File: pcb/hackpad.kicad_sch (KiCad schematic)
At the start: 39 parts, among them SW1 SW_Push, SW11 RotaryEncoder_Switch, SW2 SW_Push, SW3 SW_Push, SW4 SW_Push, SW6 SW_Push, SW7 SW_Push, SW8 SW_Push, SW9 SW_Push, U1 XIAO-RP2040-DIP

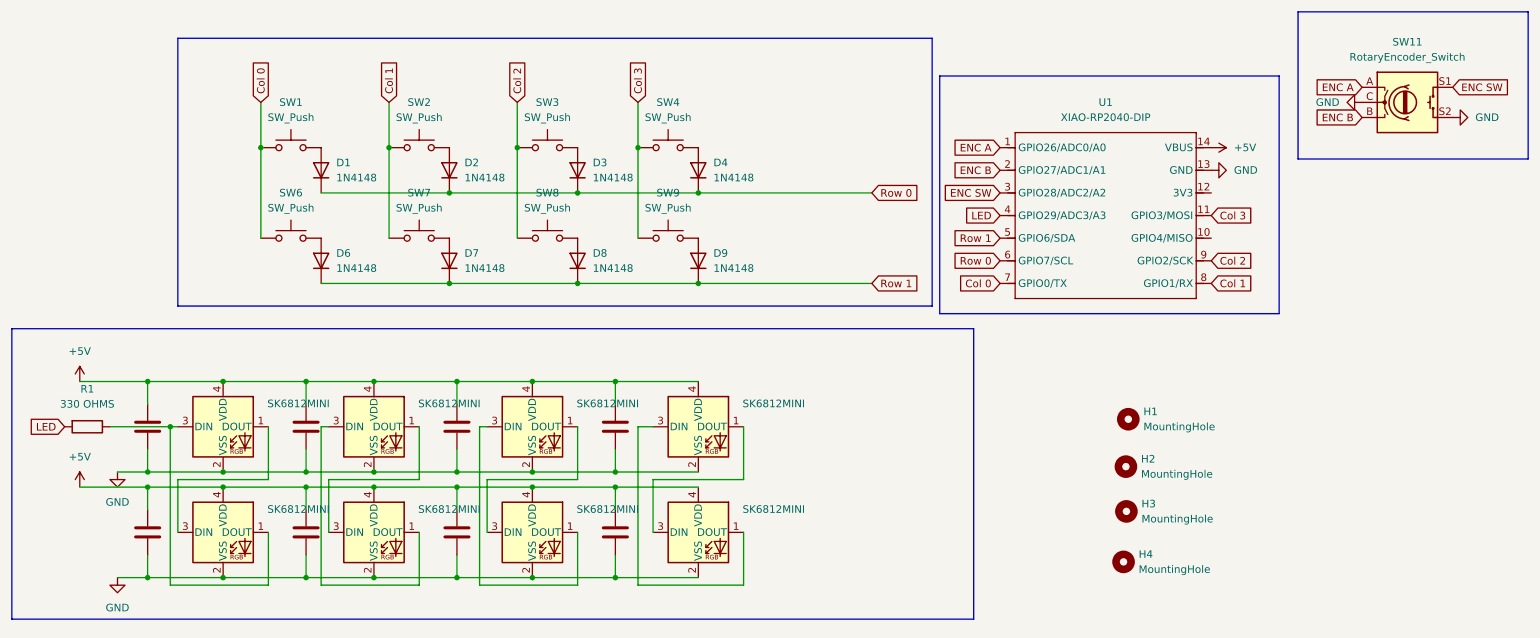
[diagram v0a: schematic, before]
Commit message: updated pcb final
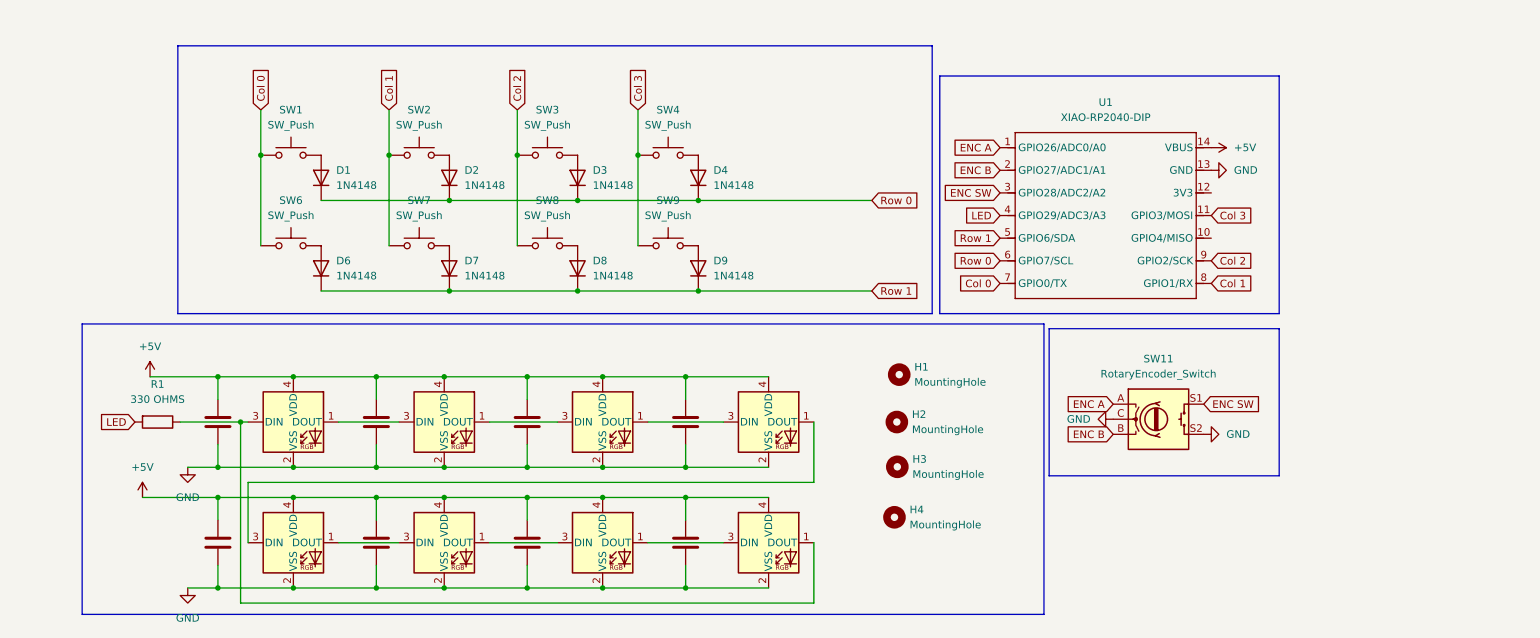
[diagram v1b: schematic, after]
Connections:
- net at D19.1 (DOUT): now also D14.3 (DIN); no longer D17.3 (DIN)
- net at D19.3 (DIN): now also D13.1 (DOUT); no longer D17.1 (DOUT)
- net at D11.1 (DOUT): now also D12.3 (DIN); no longer D14.3 (DIN)
- net at D11.3 (DIN), R1.1: now also D17.1 (DOUT); no longer D14.1 (DOUT)
- net at D16.1 (DOUT): now also D17.3 (DIN); no longer D13.3 (DIN)
- net at D16.3 (DIN): now also D15.1 (DOUT); no longer D13.1 (DOUT)
- net at D15.3 (DIN): now also D14.1 (DOUT); no longer D12.1 (DOUT)
- new net: D12.1 (DOUT), D13.3 (DIN)
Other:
- moved on the sheet: D1, D2, D3, D4, D6, D7, D8, D9, H1, H2, H3, H4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
